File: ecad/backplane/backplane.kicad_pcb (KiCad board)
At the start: 2 copper layers, 18 parts, among them J1 10145891-0320J13LF, J2 10145891-0320J13LF, J3 10145891-0320J13LF, J4 10145891-0320J13LF, J6 USB4105-GF-A, U1 MCP16331x-xCH

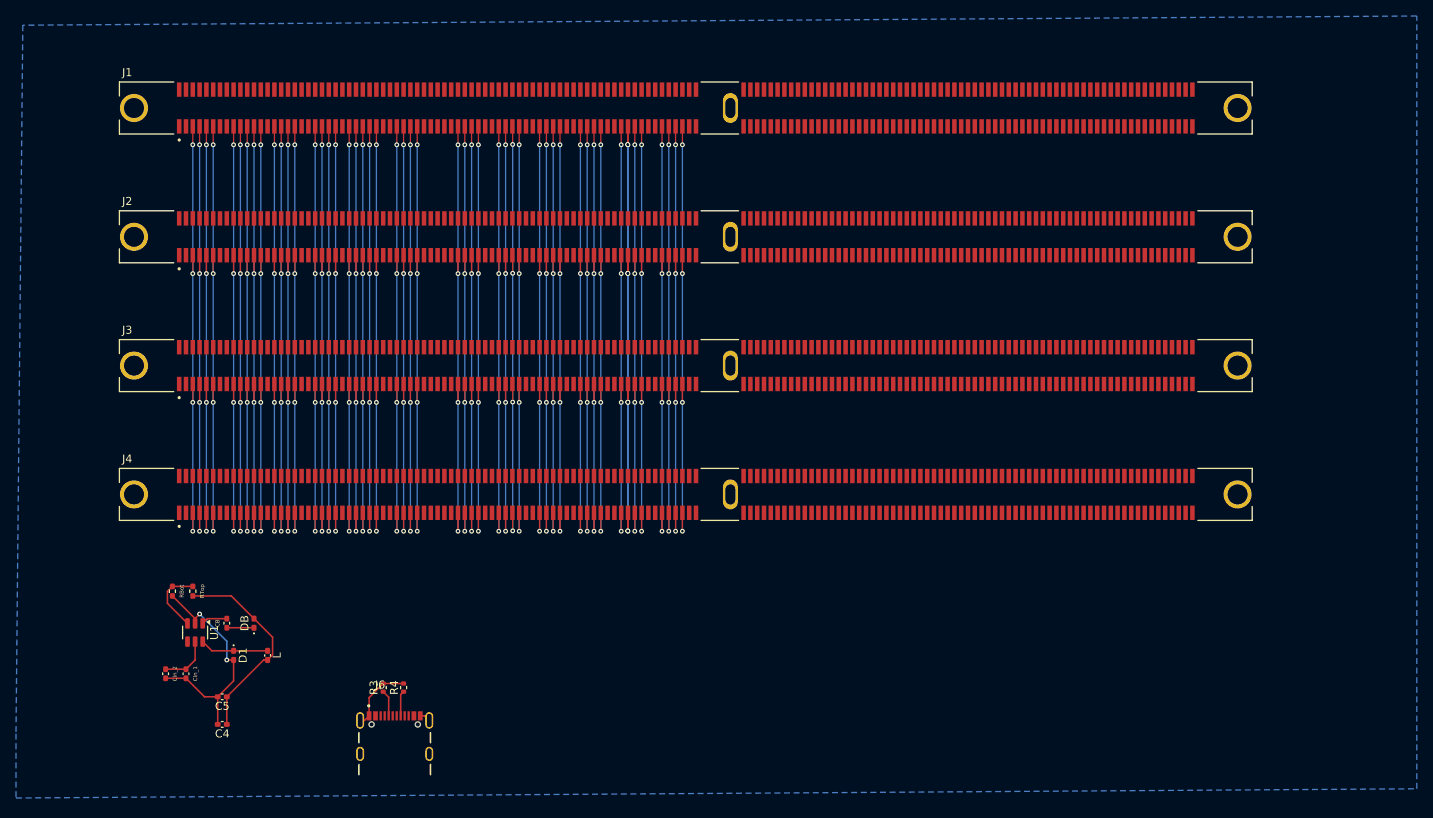
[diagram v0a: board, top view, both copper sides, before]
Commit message: hii
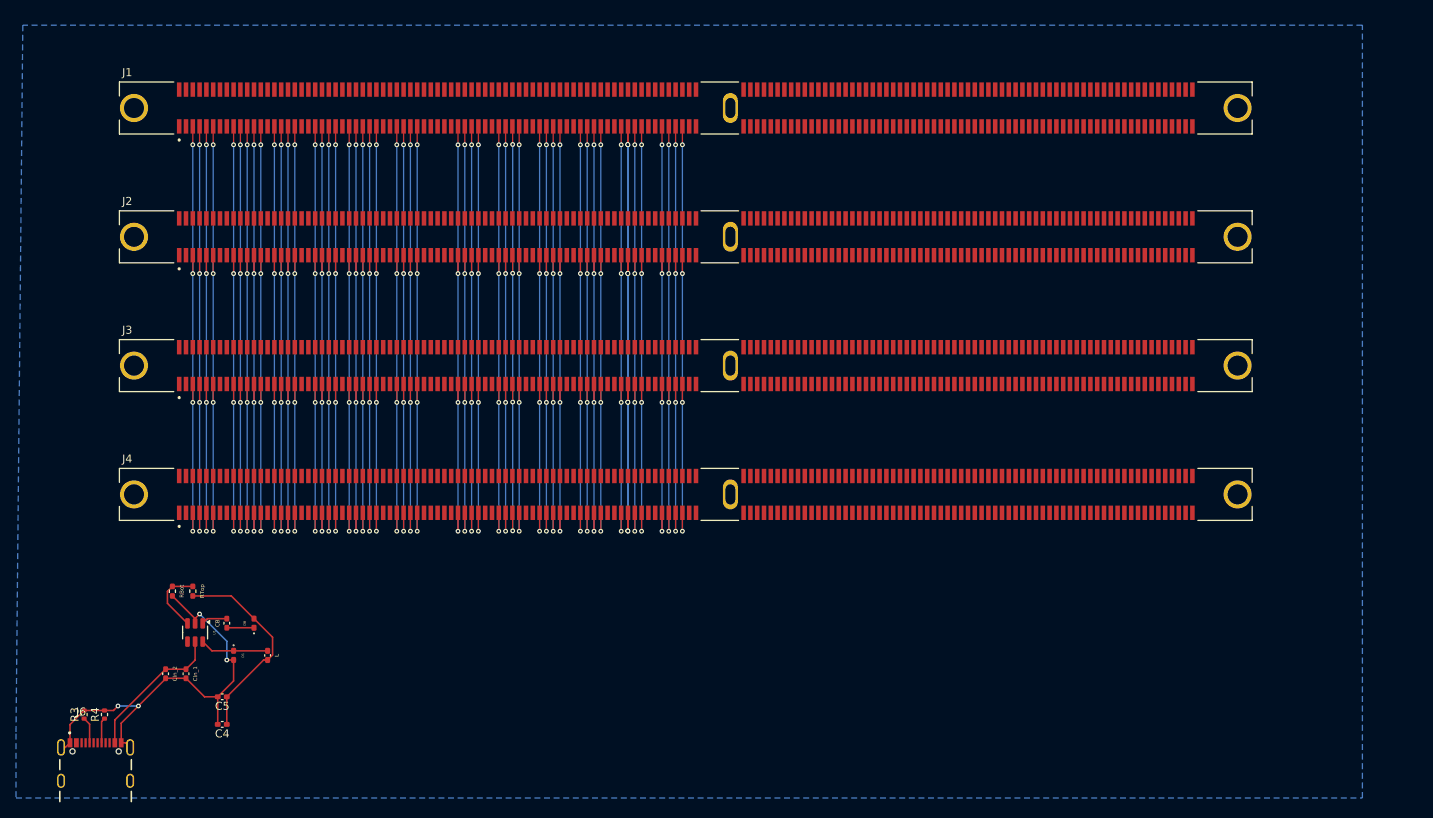
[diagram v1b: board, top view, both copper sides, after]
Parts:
- moved R4 37.5 mm to (34.0, 106.9)
- moved J6 37.5 mm to (32.9, 115.2)
- moved R3 37.5 mm to (31.5, 106.9)
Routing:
- net GND: track 97.9 -> 112.7 mm, vias 6 -> 8
- net +5V: track 6.47 -> 18.3 mm
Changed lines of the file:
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@@
 			(effects
 				(font
-					(size 1 1)
-					(thickness 0.15)
+					(size 0.5 0.5)
+					(thickness 0.125)
 				)
 			)
@@
 			(effects
 				(font
-					(size 1 1)
-					(thickness 0.15)
+					(size 0.3 0.3)
+					(thickness 0.075)
 				)
 			)
@@
 			(effects
 				(font
-					(size 1 1)
-					(thickness 0.15)
+					(size 0.3 0.3)
+					(thickness 0.075)
 				)
 			)
@@
 			(effects
 				(font
-					(size 1 1)
-					(thickness 0.15)
+					(size 0.3 0.3)
+					(thickness 0.075)
 				)
 			)
@@
 			(effects
 				(font
-					(size 1 1)
-					(thickness 0.15)
+					(size 0.3 0.3)
+					(thickness 0.075)
 				)
 			)
@@
 			(effects
 				(font
-					(size 1 1)
-					(thickness 0.15)
+					(size 0.3 0.3)
+					(thickness 0.075)
 				)
 			)
@@
 	(footprint "Resistor_SMD:R_0402_1005Metric"
 		(layer "F.Cu")
-		(at 68.85 103.5 90)
+		(at 31.4625 106.87 90)
 		(descr "Resistor SMD 0402 (1005 Metric), square (rectangular) end terminal, IPC_7351 nominal, (Body size source: IPC-SM-782 page 72, https://www.pcb-3d.com/wordpress/wp-content/uploads/ipc-sm-782a_amendment_1_and_2.pdf), generated with kicad-footprint-generator")
 		(tags "resistor")
@@
 			(effects
 				(font
-					(size 1 1)
-					(thickness 0.15)
+					(size 0.3 0.3)
+					(thickness 0.075)
 				)
 			)
@@
 			(effects
 				(font
-					(size 1 1)
-					(thickness 0.15)
+					(size 0.3 0.3)
+					(thickness 0.075)
 				)
 			)
@@
 	(footprint "Resistor_SMD:R_0402_1005Metric"
 		(layer "F.Cu")
-		(at 71.4 103.5 90)
+		(at 34.0125 106.87 90)
 		(descr "Resistor SMD 0402 (1005 Metric), square (rectangular) end terminal, IPC_7351 nominal, (Body size source: IPC-SM-782 page 72, https://www.pcb-3d.com/wordpress/wp-content/uploads/ipc-sm-782a_amendment_1_and_2.pdf), generated with kicad-footprint-generator")
 		(tags "resistor")
@@
 	(footprint "Library:GCT_USB4105-GF-A"
 		(layer "F.Cu")
-		(at 70.2875 111.785)
+		(at 32.9 115.155)
 		(property "Reference" "J6"
 			(at -1.825 -8.635 0)
@@
 	)
 	(segment
+		(start 35.3 110.4)
+		(end 35.3 107.55)
+		(width 0.2)
+		(layer "F.Cu")
+		(net 898)
+	)
+	(segment
 		(start 45.3375 100.0625)
 		(end 44.2 101.2)
@@
 	)
 	(segment
-		(start 68.85 102.99)
-		(end 71.4 102.99)
+		(start 35.3 107.55)
+		(end 41.65 101.2)
+		(width 0.2)
+		(layer "F.Cu")
+		(net 898)
+	)
+	(segment
+		(start 31.4625 106.36)
+		(end 34.0125 106.36)
 		(width 0.2)
 		(layer "F.Cu")
@@
 	)
 	(segment
-		(start 67.0875 107.03)
-		(end 67.0875 104.7525)
+		(start 29.7 110.4)
+		(end 29.7 108.1225)
+		(width 0.2)
+		(layer "F.Cu")
+		(net 899)
+	)
+	(segment
+		(start 35.14 106.36)
+		(end 35.7 105.8)
+		(width 0.2)
+		(layer "F.Cu")
+		(net 899)
+	)
+	(segment
+		(start 36.1 107.95)
+		(end 36.1 110.4)
 		(width 0.2)
 		(layer "F.Cu")
@@
 	)
 	(segment
-		(start 74.0325 107.03)
-		(end 74.6075 107.605)
+		(start 36.645 110.4)
+		(end 37.22 110.975)
+		(width 0.2)
+		(layer "F.Cu")
+		(net 899)
+	)
+	(segment
+		(start 38.25 105.8)
+		(end 41.65 102.4)
 		(width 0.2)
 		(layer "F.Cu")
@@
 	)
 	(segment
-		(start 67.0875 104.7525)
-		(end 68.85 102.99)
+		(start 29.7 108.1225)
+		(end 31.4625 106.36)
 		(width 0.2)
 		(layer "F.Cu")
@@
 	)
 	(segment
-		(start 65.9675 107.605)
-		(end 66.5125 107.605)
+		(start 28.58 110.975)
+		(end 29.125 110.975)
 		(width 0.2)
 		(layer "F.Cu")
@@
 	)
 	(segment
-		(start 73.4875 107.03)
-		(end 74.0325 107.03)
+		(start 36.1 110.4)
+		(end 36.645 110.4)
 		(width 0.2)
 		(layer "F.Cu")
@@
 	)
 	(segment
+		(start 41.65 102.4)
+		(end 41.65 102.335)
+		(width 0.2)
+		(layer "F.Cu")
+		(net 899)
+	)
+	(segment
 		(start 46.515 104.65)
 		(end 44.2 102.335)
@@
 	)
 	(segment
-		(start 66.5125 107.605)
-		(end 67.0875 107.03)
+		(start 38.25 105.8)
+		(end 36.1 107.95)
+		(width 0.2)
+		(layer "F.Cu")
+		(net 899)
+	)
+	(segment
+		(start 34.0125 106.36)
+		(end 35.14 106.36)
+		(width 0.2)
+		(layer "F.Cu")
+		(net 899)
+	)
+	(segment
+		(start 29.125 110.975)
+		(end 29.7 110.4)
 		(width 0.2)
 		(layer "F.Cu")
@@
 	)
 	(via
+		(at 38.25 105.8)
+		(size 0.6)
+		(drill 0.3)
+		(layers "F.Cu" "B.Cu")
+		(net 899)
+	)
+	(via
 		(at 49.3 100.05)
 		(size 0.6)
@@
 	)
 	(via
+		(at 35.7 105.8)
+		(size 0.6)
+		(drill 0.3)
+		(layers "F.Cu" "B.Cu")
+		(net 899)
+	)
+	(via
 		(at 64.6 83.95)
 		(size 0.6)
@@
 	)
 	(segment
+		(start 35.7 105.8)
+		(end 38.25 105.8)
+		(width 0.2)
+		(layer "B.Cu")
+		(net 899)
+	)
+	(segment
 		(start 64.6 35.65)
 		(end 64.6 51.75)
@@
 	)
 	(segment
-		(start 69.5375 107.03)
-		(end 69.5375 104.6975)
+		(start 32.15 110.4)
+		(end 32.15 108.0675)
 		(width 0.2)
 		(layer "F.Cu")
@@
 	)
 	(segment
-		(start 69.5375 104.6975)
-		(end 68.85 104.01)
+		(start 32.15 108.0675)
+		(end 31.4625 107.38)
 		(width 0.2)
 		(layer "F.Cu")
@@
 	)
 	(segment
-		(start 71.0375 107.03)
-		(end 71.0375 104.3725)
+		(start 33.65 110.4)
+		(end 33.65 107.7425)
 		(width 0.2)
 		(layer "F.Cu")
@@
 	)
 	(segment
-		(start 71.0375 104.3725)
-		(end 71.4 104.01)
+		(start 33.65 107.7425)
+		(end 34.0125 107.38)
 		(width 0.2)
 		(layer "F.Cu")
@@
 		(min_thickness 0.25)
 		(filled_areas_thickness no)
-		(fill yes
+		(fill
 			(thermal_gap 0.5)
 			(thermal_bridge_width 0.5)
@@
 		(polygon
 			(pts
-				(xy 198.05 19.55) (xy 23.8 20.7) (xy 22.95 109.25) (xy 22.95 117.3) (xy 198.05 116.15)
+				(xy 191.25 20.7) (xy 23.8 20.7) (xy 22.95 109.25) (xy 22.95 117.3) (xy 191.25 117.3)
 			)
 		)
